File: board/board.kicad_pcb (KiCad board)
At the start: 2 copper layers, 21 x 13 mm, 1 part

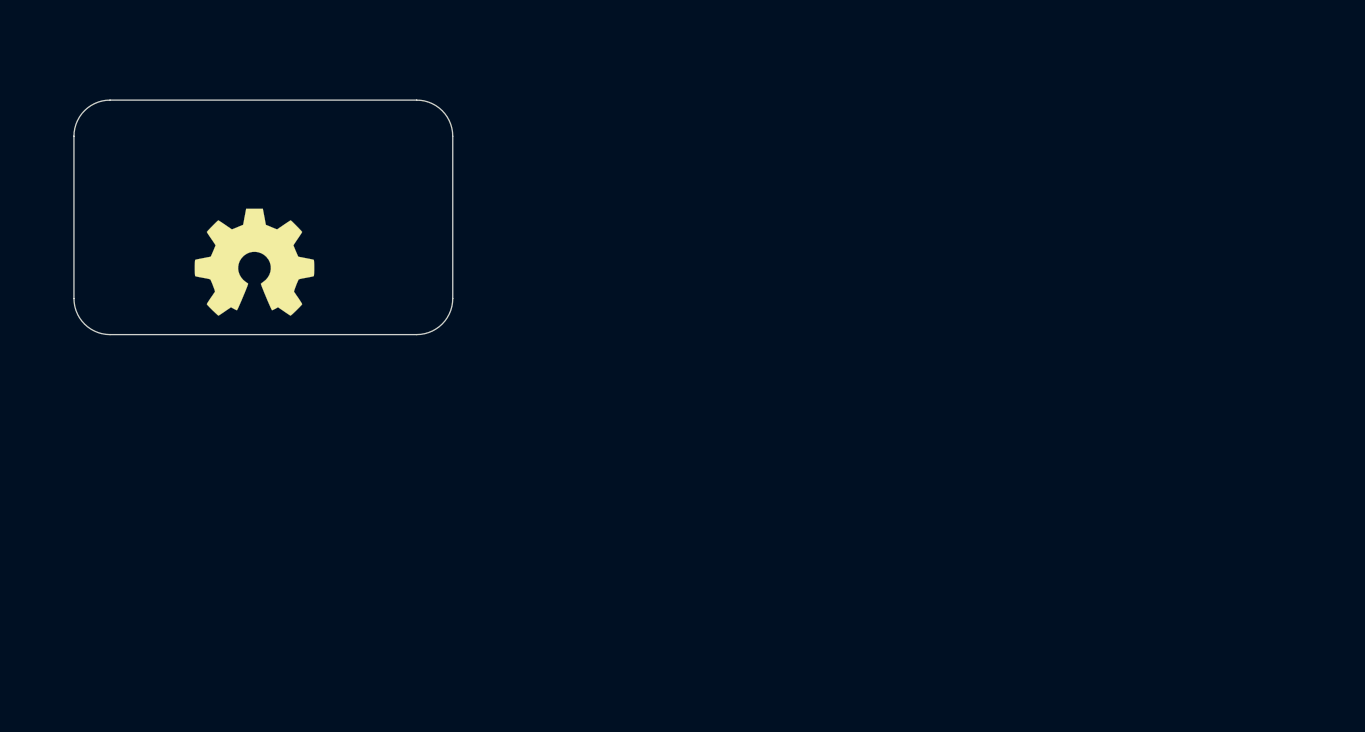
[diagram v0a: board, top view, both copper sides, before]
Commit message: initial
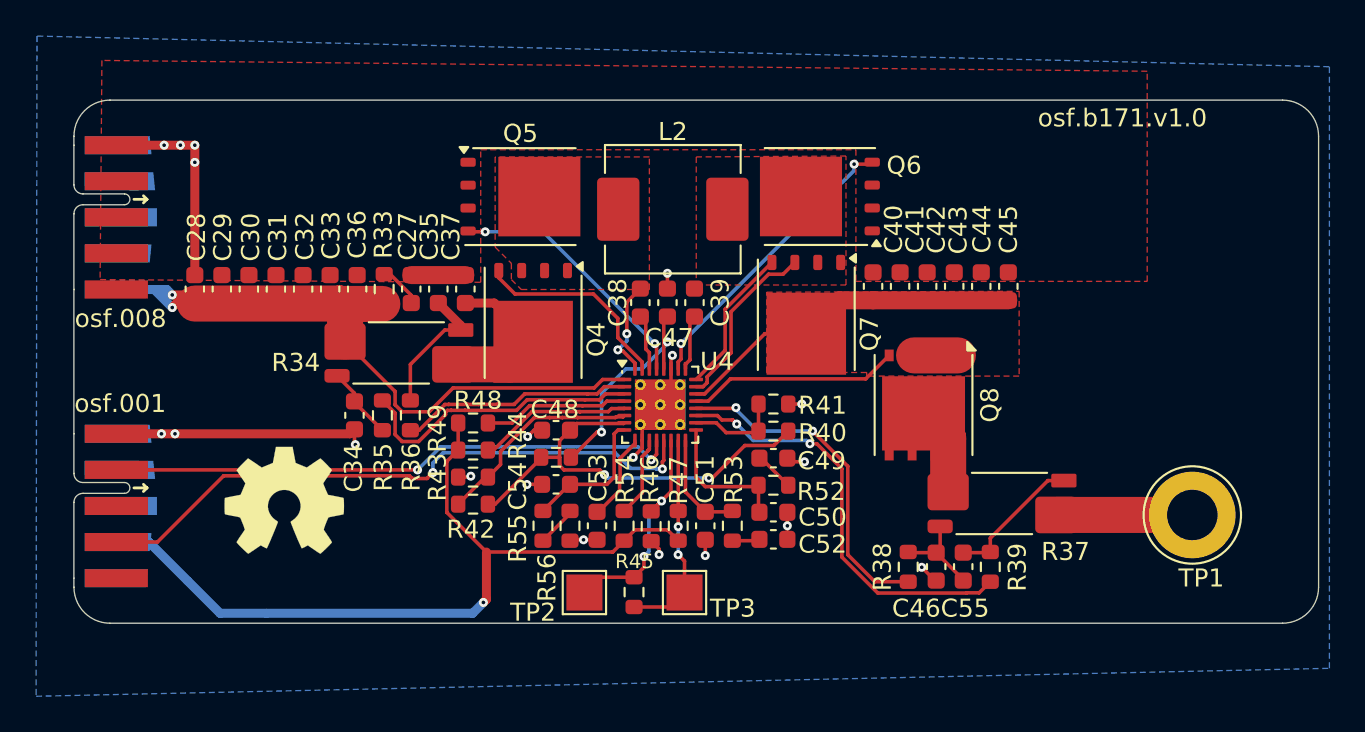
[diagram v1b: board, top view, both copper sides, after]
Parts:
- added C27: 1uF, Capacitor_SMD:C_0603_1608Metric, F.Cu at (158.7, 100.5)
- added C28: 10uF, Capacitor_SMD:C_0603_1608Metric, F.Cu at (146.7, 100.5)
- added C29: 10uF, Capacitor_SMD:C_0603_1608Metric, F.Cu at (148.2, 100.5)
- added C30: 10uF, Capacitor_SMD:C_0603_1608Metric, F.Cu at (149.7, 100.5)
- added C31: 10uF, Capacitor_SMD:C_0603_1608Metric, F.Cu at (151.2, 100.5)
- added C32: 10uF, Capacitor_SMD:C_0603_1608Metric, F.Cu at (152.7, 100.5)
- added C33: 10uF, Capacitor_SMD:C_0603_1608Metric, F.Cu at (154.2, 100.5)
- added C34: 33nF, Capacitor_SMD:C_0603_1608Metric, F.Cu at (155.6, 107.5)
- added C35: 33nF, Capacitor_SMD:C_0603_1608Metric, F.Cu at (160.2, 100.5)
- added C36: 470nF, Capacitor_SMD:C_0603_1608Metric, F.Cu at (155.7, 100.5)
- added C37: 10nF, Capacitor_SMD:C_0603_1608Metric, F.Cu at (161.7, 100.5)
- added C38: 47nF, Capacitor_SMD:C_0603_1608Metric, F.Cu at (171.4, 101.2)
- added C39: 47nF, Capacitor_SMD:C_0603_1608Metric, F.Cu at (174.4, 101.2)
- added C40: 10uF, Capacitor_SMD:C_0603_1608Metric, F.Cu at (184.3, 100.3)
- added C41: 10uF, Capacitor_SMD:C_0603_1608Metric, F.Cu at (185.8, 100.3)
- added C42: 10uF, Capacitor_SMD:C_0603_1608Metric, F.Cu at (187.3, 100.3)
- added C43: 10uF, Capacitor_SMD:C_0603_1608Metric, F.Cu at (188.8, 100.3)
- added C44: 10uF, Capacitor_SMD:C_0603_1608Metric, F.Cu at (190.3, 100.3)
- added C45: 10uF, Capacitor_SMD:C_0603_1608Metric, F.Cu at (191.8, 100.3)
- added C46: 1uF, Capacitor_SMD:C_0603_1608Metric, F.Cu at (187.8, 115.9)
- added C47: 2.2uF, Capacitor_SMD:C_0603_1608Metric, F.Cu at (172.9, 101.2)
- added C48: 1uF, Capacitor_SMD:C_0603_1608Metric, F.Cu at (166.7, 108.3)
- added C49: 680pF, Capacitor_SMD:C_0603_1608Metric, F.Cu at (178.8, 109.8)
- added C50: 15pF, Capacitor_SMD:C_0603_1608Metric, F.Cu at (178.8, 112.8)
- added C51: 33pF, Capacitor_SMD:C_0603_1608Metric, F.Cu at (175.0, 113.6)
- added C52: 1800pF, Capacitor_SMD:C_0603_1608Metric, F.Cu at (178.8, 114.3)
- added C53: 100pF, Capacitor_SMD:C_0603_1608Metric, F.Cu at (169.0, 113.6)
- added C54: 100pF, Capacitor_SMD:C_0603_1608Metric, F.Cu at (166.7, 111.3)
- added C55: 0.1uF, Capacitor_SMD:C_0603_1608Metric, F.Cu at (189.3, 115.9)
- added J1: 001_I2C, on_edge:on_edge_2x05_device, F.Cu at (140.0, 112.5)
- added J2: 008_USB, on_edge:on_edge_2x05_device, F.Cu at (140.0, 96.5)
- added L2: MWSA0603S-2R2MT, Inductor_SMD:L_Sunlord_MWSA0603S, F.Cu at (173.2, 96.0)
- added Q4: CSD18534Q5A, Package_TO_SOT_SMD:TDSON-8-1, F.Cu at (165.5, 102.3)
- added Q5: CSD18534Q5A, Package_TO_SOT_SMD:TDSON-8-1, F.Cu at (164.8, 95.3)
- added Q6: CSD18534Q5A, Package_TO_SOT_SMD:TDSON-8-1, F.Cu at (181.4, 95.3)
- added Q7: CSD18534Q5A, Package_TO_SOT_SMD:TDSON-8-1, F.Cu at (180.6, 101.9)
- added Q8: AON6411, Package_DFN_QFN:AO_DFN-8-1EP_5.55x5.2mm_P1.27mm_EP4.12x4.6mm, F.Cu at (187.1, 106.9)
- added R33: 2.2R, Resistor_SMD:R_0603_1608Metric, F.Cu at (157.2, 100.5)
- added R34: 10mΩ SHUNT FMF25FPJR010-LH, Resistor_SMD:R_Shunt_Vishay_WSK2512_6332Metric_T1.19mm, F.Cu at (158.0, 104.0)
- added R35: 5.1R, Resistor_SMD:R_0603_1608Metric, F.Cu at (157.1, 107.5)
- added R36: 5.1R, Resistor_SMD:R_0603_1608Metric, F.Cu at (158.7, 107.5)
- added R37: 10mΩ SHUNT FMF25FPJR010-LH, Resistor_SMD:R_Shunt_Vishay_WSK2512_6332Metric_T1.19mm, F.Cu at (191.4, 112.4)
- added R38: 10R, Resistor_SMD:R_0603_1608Metric, F.Cu at (186.2, 115.9)
- added R39: 10R, Resistor_SMD:R_0603_1608Metric, F.Cu at (190.8, 115.9)
- added R40: 130k, Resistor_SMD:R_0603_1608Metric, F.Cu at (178.8, 108.3)
- added R41: 470k, Resistor_SMD:R_0603_1608Metric, F.Cu at (178.8, 106.8)
- added R42: 390k, Resistor_SMD:R_0603_1608Metric, F.Cu at (162.1, 112.4)
- added R43: 220k, Resistor_SMD:R_0603_1608Metric, F.Cu at (162.1, 110.9)
- added R44: 10R, Resistor_SMD:R_0603_1608Metric, F.Cu at (166.7, 109.8)
- added R45: 2M, Resistor_SMD:R_0603_1608Metric, F.Cu at (171.1, 117.3)
- added R46: 300k, Resistor_SMD:R_0603_1608Metric, F.Cu at (172.0, 113.6)
- added R47: 10k, Resistor_SMD:R_0603_1608Metric, F.Cu at (173.5, 113.6)
- added R48: 10k, Resistor_SMD:R_0603_1608Metric, F.Cu at (162.1, 107.9)
- added R49: 10k, Resistor_SMD:R_0603_1608Metric, F.Cu at (162.1, 109.4)
- added R52: 10k, Resistor_SMD:R_0603_1608Metric, F.Cu at (178.8, 111.3)
- added R53: 40.2k, Resistor_SMD:R_0603_1608Metric, F.Cu at (176.5, 113.6)
- added R54: 200R, Resistor_SMD:R_0603_1608Metric, F.Cu at (170.5, 113.6)
- added R55: 110k, Resistor_SMD:R_0603_1608Metric, F.Cu at (166.0, 113.6)
- added R56: 27k, Resistor_SMD:R_0603_1608Metric, F.Cu at (167.5, 113.6)
- added TP1: TestPoint, TestPoint:TestPoint_Loop_D3.80mm_Drill2.8mm, F.Cu at (202.0, 113.0)
- added TP2: CMPIN, TestPoint:TestPoint_Pad_2.0x2.0mm, F.Cu at (168.3, 117.3)
- added TP3: CMPOUT, TestPoint:TestPoint_Pad_2.0x2.0mm, F.Cu at (173.8, 117.3)
- added U4: BQ25713RSNR, Package_DFN_QFN:Texas_RSN_WQFN-32-1EP_4x4mm_P0.4mm_EP2.8x2.8mm_ThermalVias, F.Cu at (172.5, 106.9)
- moved LOGO1 13.3 mm to (151.7, 112.2)
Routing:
- net GND: track 0.00 -> 46.3 mm, vias 0 -> 20
- net /charger/V3.3: track 0.00 -> 44.8 mm, vias 0 -> 1
- net /charger/VBUS: track 0.00 -> 38.6 mm, vias 0 -> 2
- net /charger/SCL: track 0.00 -> 34.7 mm, vias 0 -> 2
- net /charger/SDA: track 0.00 -> 31.7 mm, vias 0 -> 2
- net /charger/VDDA: track 0.00 -> 25.0 mm, vias 0 -> 2
- net /charger/SRN: track 0.00 -> 23.5 mm, vias 0 -> 2
- net /charger/VSYS: track 0.00 -> 21.9 mm
- net /charger/SRP: track 0.00 -> 18.7 mm, vias 0 -> 2
- net /charger/LODRV2: track 0.00 -> 16.4 mm, vias 0 -> 2
- net Net-(U4-ACP): track 0.00 -> 16.2 mm
- net /charger/LODRV1: track 0.00 -> 14.4 mm, vias 0 -> 2
- net Net-(U4-CMPIN): track 0.00 -> 13.2 mm, vias 0 -> 2
- net Net-(U4-ACN): track 0.00 -> 12.9 mm
- net /charger/REGN: track 0.00 -> 12.3 mm, vias 0 -> 2
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- added copper zone on F.Cu, net /charger/SW1
- added copper zone on F.Cu, net /charger/SW2
- added copper zone on F.Cu, net /charger/VSYS
- added copper zone on B.Cu, net GND
- added copper zone on F.Cu, net GND
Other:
- board size 21 x 13 mm -> 69 x 29 mm
- board text added: "osf.001"
- board text added: "osf.008"
- board text added: "osf.b171.v1.0"
